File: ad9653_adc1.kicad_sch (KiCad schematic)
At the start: 20 parts, among them J701 142-0701-201, J702 142-0701-201, J703 142-0701-201, J704 142-0701-201, U701 AD9653BCPZ-125

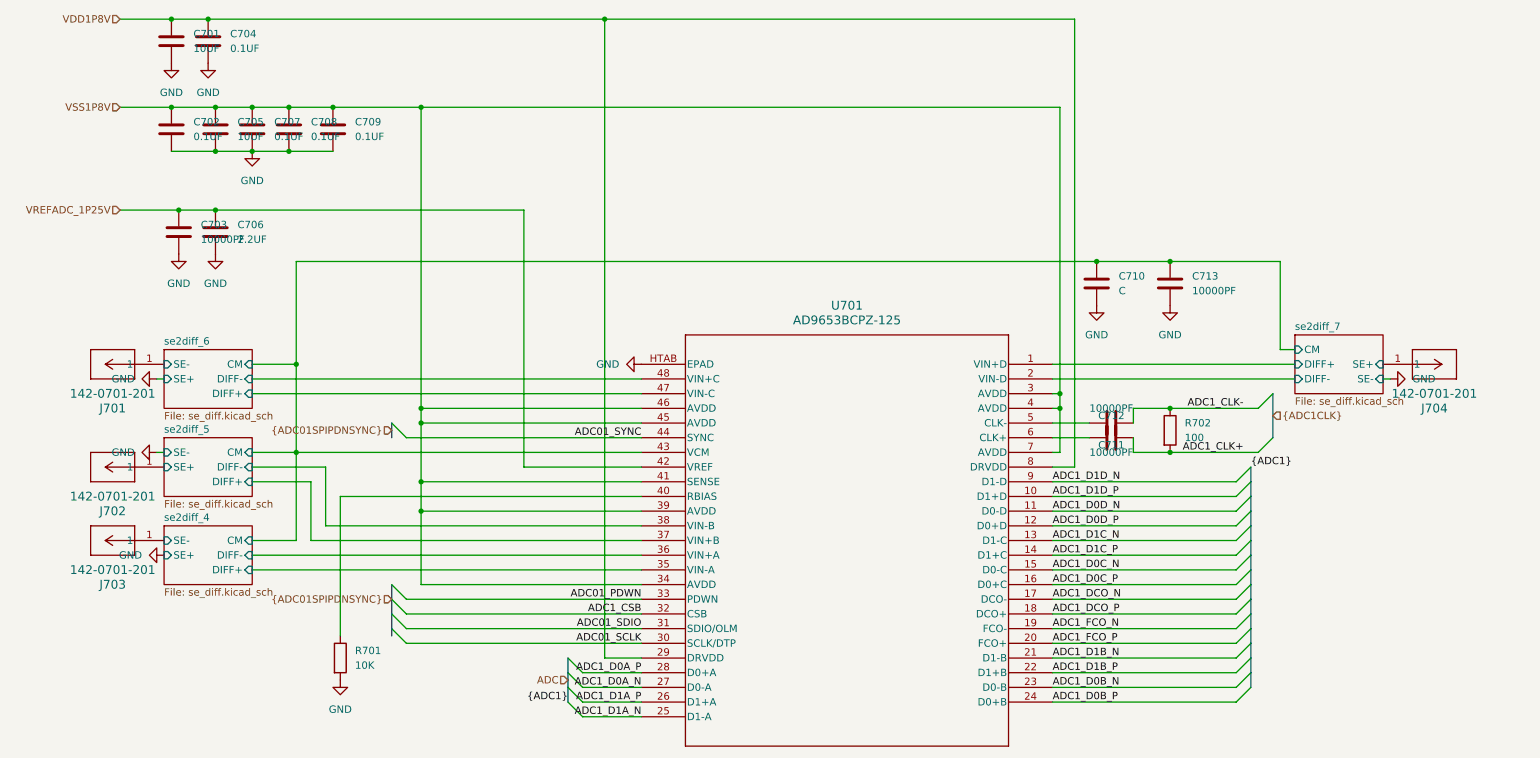
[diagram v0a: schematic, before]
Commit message: lots small updates
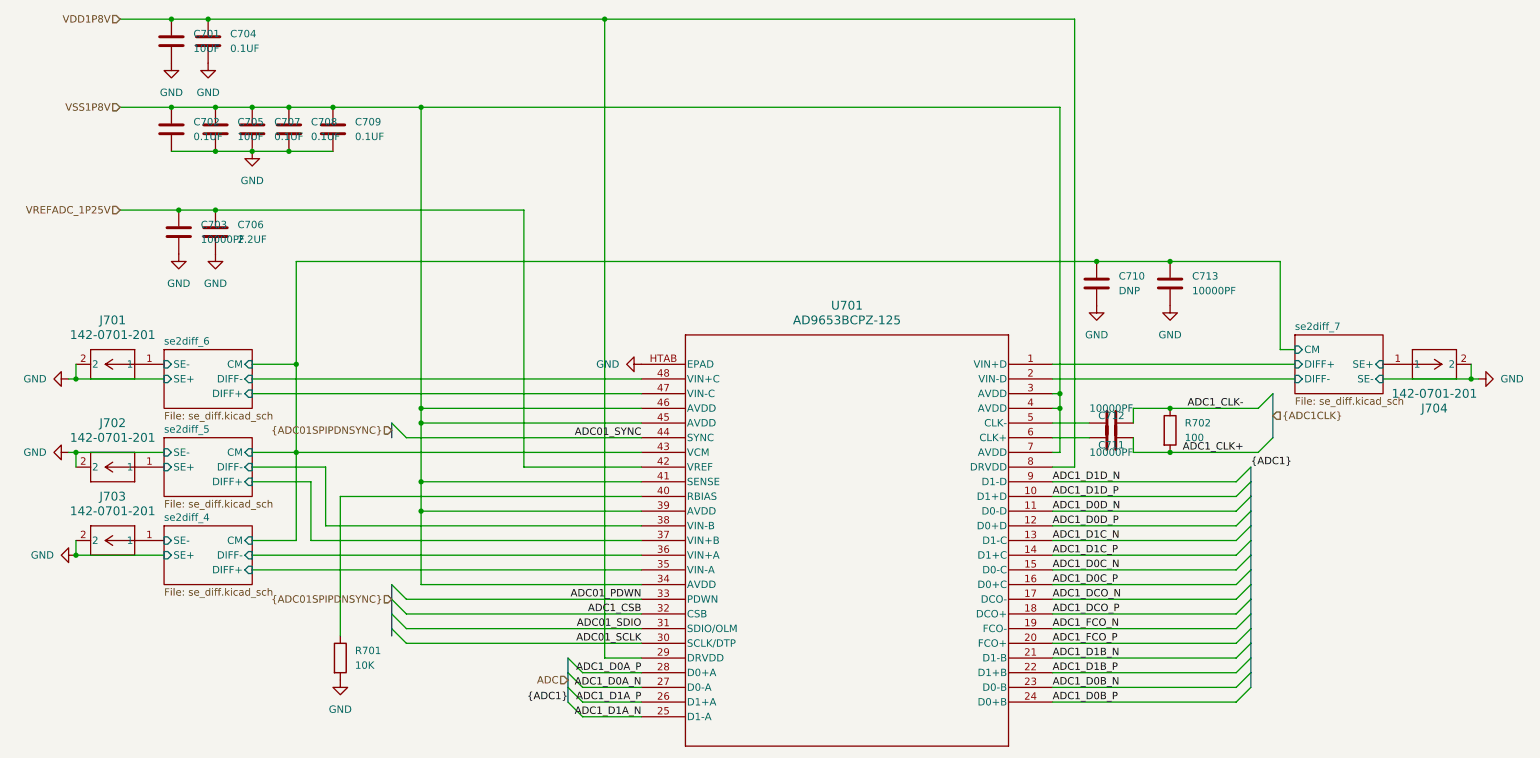
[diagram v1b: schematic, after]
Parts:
- C710: value C -> DNP
- J701, J702, J703, J704: footprint 001_download:CONN_142-0701-201_CIN -> CONN_142-0701-201_CIN; symbol 001_symbol:142-0701-201 -> 001_symbol:142-0701-201_GH
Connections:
- net GND: now also J701.2, J701.3, J701.4, J701.5, J702.2, J702.3, J702.4, J702.5, J703.2, J703.3, J703.4, J703.5, J704.2, J704.3, J704.4, J704.5
